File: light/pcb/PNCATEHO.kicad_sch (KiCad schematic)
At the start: 49 parts, among them J1 USB_C_Receptacle_USB2.0, SW11 Boot, U1 RP2040, U2 RT9013-33GB, U3 W25Q32JVSSIQ, U4 USBLC6-2SC6, Y1 12MHz

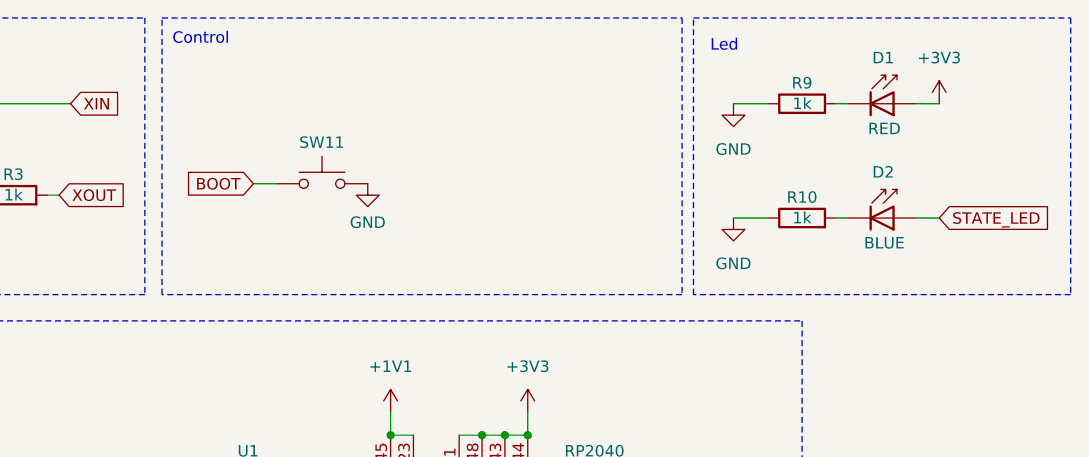
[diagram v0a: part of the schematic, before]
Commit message: remove led
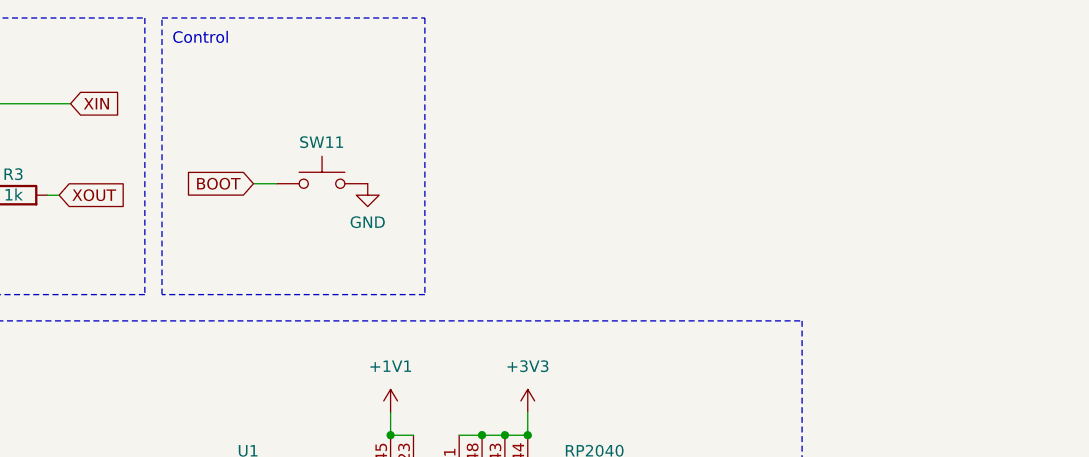
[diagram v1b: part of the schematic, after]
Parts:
- removed D1: RED, PNCATEHO:LED_0805_2012Metric_Pad1.15x1.40mm_HandSolder, symbol PNCATEHO:D_Generic
- removed D2: BLUE, PNCATEHO:LED_0805_2012Metric_Pad1.15x1.40mm_HandSolder, symbol PNCATEHO:D_Generic
- removed R10, R9: 1k, PNCATEHO:R_0805_2012Metric_Pad1.20x1.40mm_HandSolder, symbol PNCATEHO:R
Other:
- note removed: "Led"

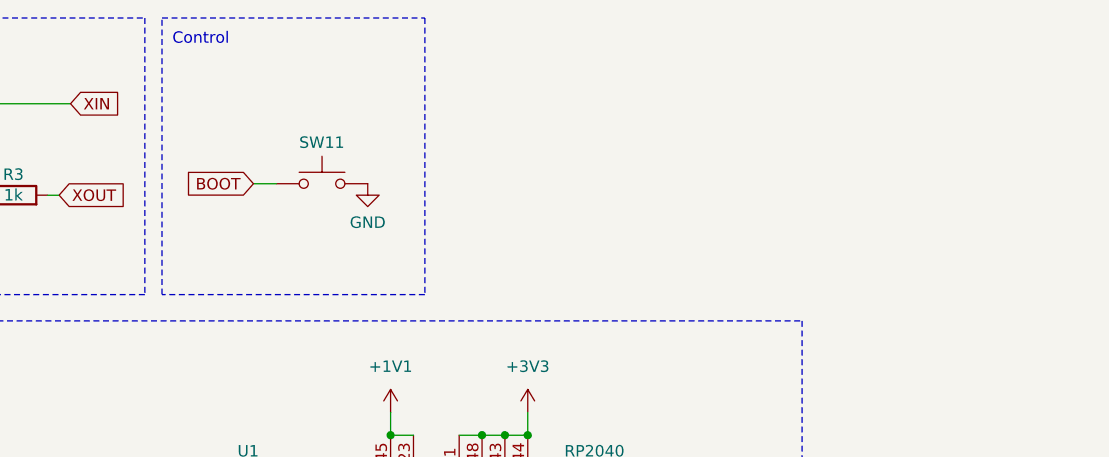
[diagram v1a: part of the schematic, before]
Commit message: fix
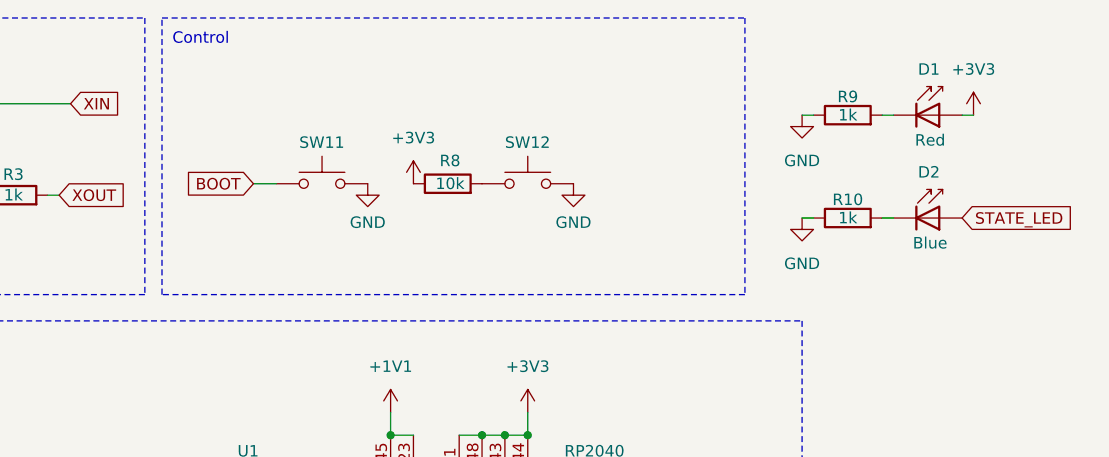
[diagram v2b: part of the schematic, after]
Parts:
- added D1: Red, PNCATEHO:D_0805_2012Metric_Pad1.15x1.40mm_HandSolder, symbol PNCATEHO:D_Generic
- added D2: Blue, PNCATEHO:D_0805_2012Metric_Pad1.15x1.40mm_HandSolder, symbol PNCATEHO:D_Generic
- added R10, R9: 1k, PNCATEHO:R_0805_2012Metric_Pad1.20x1.40mm_HandSolder, symbol PNCATEHO:R
- added R8: 10k, PNCATEHO:R_0805_2012Metric_Pad1.20x1.40mm_HandSolder, symbol PNCATEHO:R
- added SW12: Boot, PNCATEHO:PADS, symbol PNCATEHO:SW_Push
- SW11: footprint PNCATEHO:SW_SMD_L4_W3_H1.5 -> PNCATEHO:PADS
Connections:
- net +3V3: now also D1.2 (A), R8.1
- net GND: now also R10.1, R9.1, SW12.1
- net STATE_LED: now also D2.2 (A)
- new net: D1.1 (K), R9.2
- new net: R8.2, SW12.2
- new net: D2.1 (K), R10.2
